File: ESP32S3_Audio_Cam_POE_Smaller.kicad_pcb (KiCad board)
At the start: 4 copper layers, 83.2 x 32.4 mm, 50 parts, among them CN1 PJ-316C-6A, J1 Conn_01x20_Pin, J10 Conn_01x02, J2 Conn_01x20_Pin, U11 TM1637, U15 MAX98357AETE+T, U16 ICS-43434, U17 ICS-43434

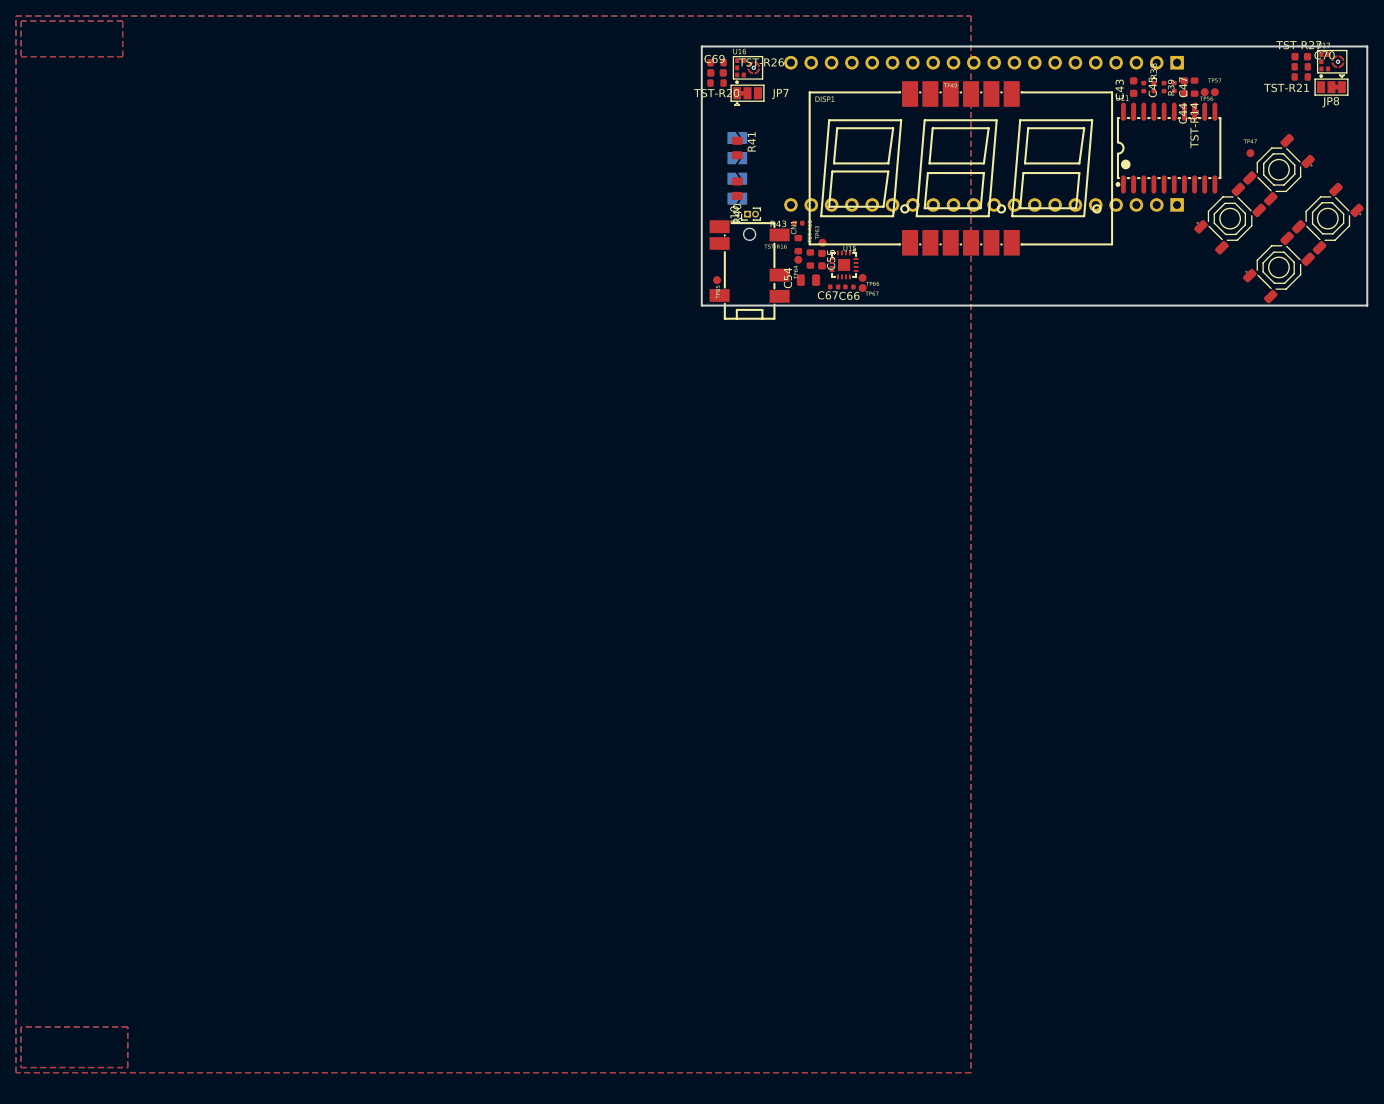
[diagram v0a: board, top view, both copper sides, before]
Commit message: Draft smaller board.
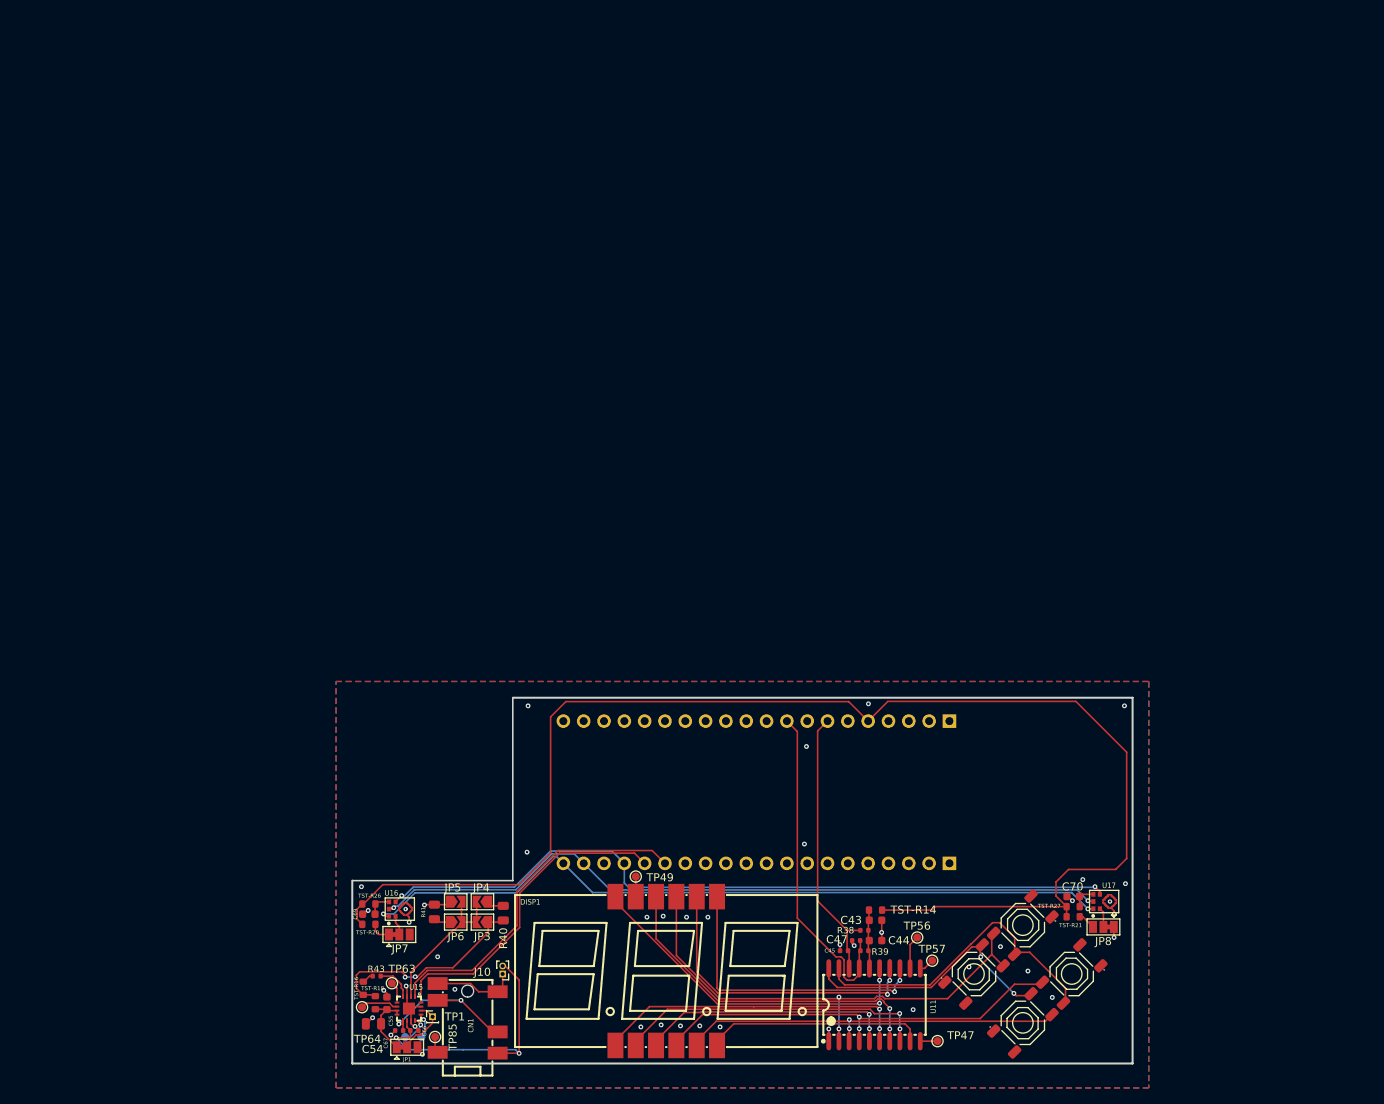
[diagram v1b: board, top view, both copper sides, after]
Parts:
- added JP1: SolderJumper_3_Bridged12, Jumper:SolderJumper-3_P1.3mm_Bridged12_Pad1.0x1.5mm, F.Cu at (89.5, 159.4)
- added TP1: TestPoint, Connector_PinHeader_1.00mm:PinHeader_1x01_P1.00mm_Vertical, F.Cu at (92.7, 155.6)
- JP3, JP4, JP5, JP6: moved to F.Cu
- TP47, TP49, TP56, TP57, TP63, TP64, TP85: footprint Project-specific:TestPoint_Pad_D1.0mm -> TestPoint:TestPoint_Pad_D1.0mm
- TP66, TP67: footprint Project-specific:TestPoint_Pad_D1.0mm -> TestPoint:TestPoint_Pad_D1.0mm; moved to B.Cu
- moved TP47 117.7 mm to (155.8, 158.6)
- moved C45 114.3 mm to (144.1, 147.3), turned to 0 degrees
- moved R39 114.3 mm to (146.7, 147.3), turned to 0 degrees
- moved TP57 114.2 mm to (155.2, 148.6)
- moved C47 113.8 mm to (145.7, 146.1), turned to 0 degrees
- moved U16 113.8 mm to (88.6, 142.1)
- moved C69 113.8 mm to (84.7, 142.8)
- moved JP7 113.8 mm to (88.6, 145.3)
- moved TST-R20 113.8 mm to (84.7, 144.0)
- moved TST-R26 113.8 mm to (84.7, 141.5)
- moved C44 113.5 mm to (148.1, 146.1), turned to 0 degrees
- moved U11 113.2 mm to (148.0, 154.1)
- moved TP56 111.6 mm to (153.3, 145.7)
- moved R38 111.5 mm to (146.7, 144.8), turned to 0 degrees
- moved TST-R14 110.3 mm to (148.1, 142.2), turned to 0 degrees
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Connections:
- net Net-(C54-Pad1) renamed /V.SPK
- J1 pad 15: /SPK.BCLK -> /SPK.DIN
- J1 pad 16: /SPK.DIN -> /SPK.BCLK
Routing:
- net +3V3: track 0.00 -> 175.2 mm
- net /MIC.WS: track 0.00 -> 95.3 mm, vias 0 -> 2
- net /MIC.SCK: track 0.00 -> 94.6 mm, vias 0 -> 2
- net /MIC.SD: track 0.00 -> 93.4 mm, vias 0 -> 2
- net /7SEG.SEG1: track 0.00 -> 62.0 mm, vias 0 -> 2
- net /7SEG.SEG3: track 0.00 -> 52.9 mm, vias 0 -> 2
- net /7SEG.SEG2: track 0.00 -> 49.3 mm, vias 0 -> 2
- net /7SEG.GRID1: track 0.00 -> 43.4 mm, vias 0 -> 2
- net /SPK.DIN: track 0.00 -> 43.0 mm
- net /7SEG.SEG6: track 0.00 -> 42.5 mm, vias 0 -> 2
- net /7SEG.DIO: track 0.00 -> 42.0 mm
- net /SPK.BCLK: track 0.00 -> 40.3 mm
- net /7SEG.K1: track 0.00 -> 40.0 mm
- net /7SEG.SEG5: track 0.00 -> 39.5 mm, vias 0 -> 2
- net /7SEG.SEG7: track 0.00 -> 38.9 mm, vias 0 -> 2
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- removed copper zone on In2.Cu, net (none)
- removed copper zone on In2.Cu, net +3V3
- removed copper zone on In1.Cu, net COM
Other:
- board size 83.2 x 32.4 mm -> 97.5 x 45.7 mm
- copper layers 4 -> 2
